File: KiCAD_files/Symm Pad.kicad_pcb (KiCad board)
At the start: 2 copper layers, 21 parts, among them J1 0.91"_OLED_Display, SW1 SW_Push, SW2 SW_Push, SW3 SW_Push, SW4 SW_Push, SW5 SW_Push, SW6 SW_Push, SW7 RotaryEncoder_Switch, U1 XIAO-RP2040-DIP

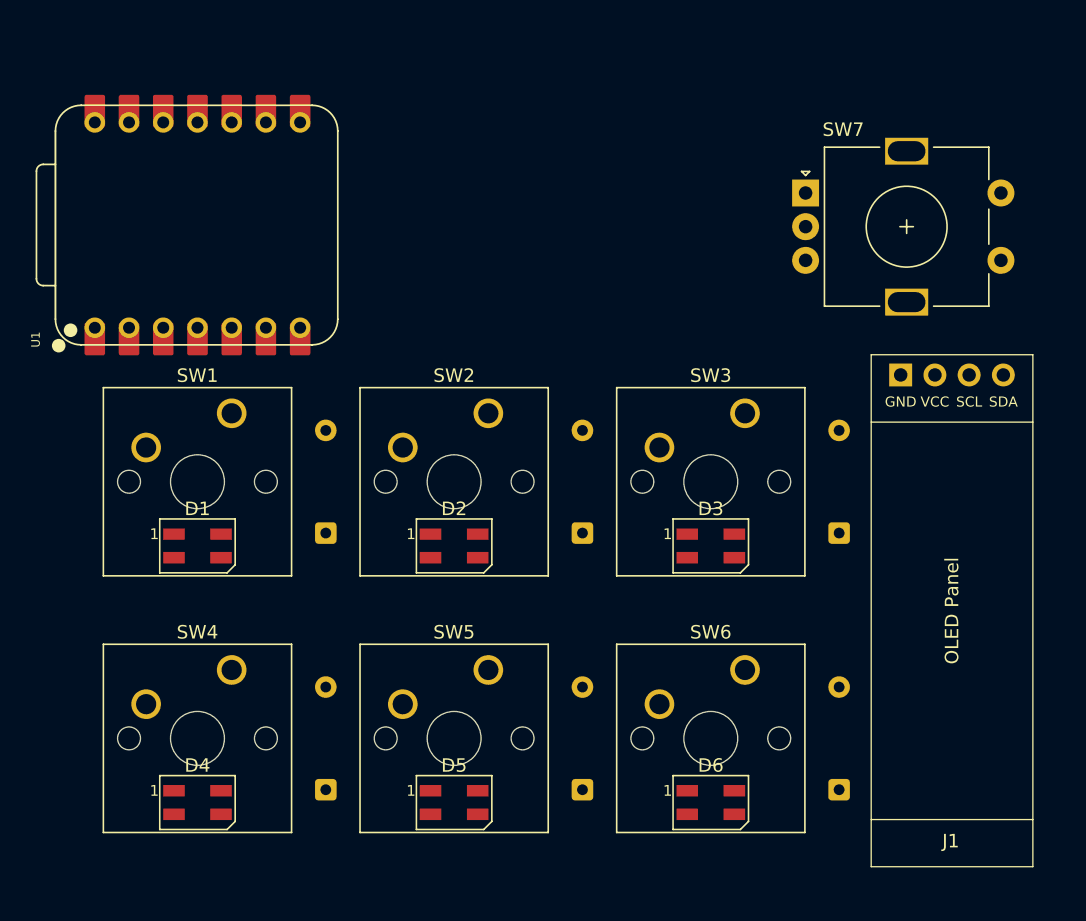
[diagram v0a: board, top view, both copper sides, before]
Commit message: Completed the PCB
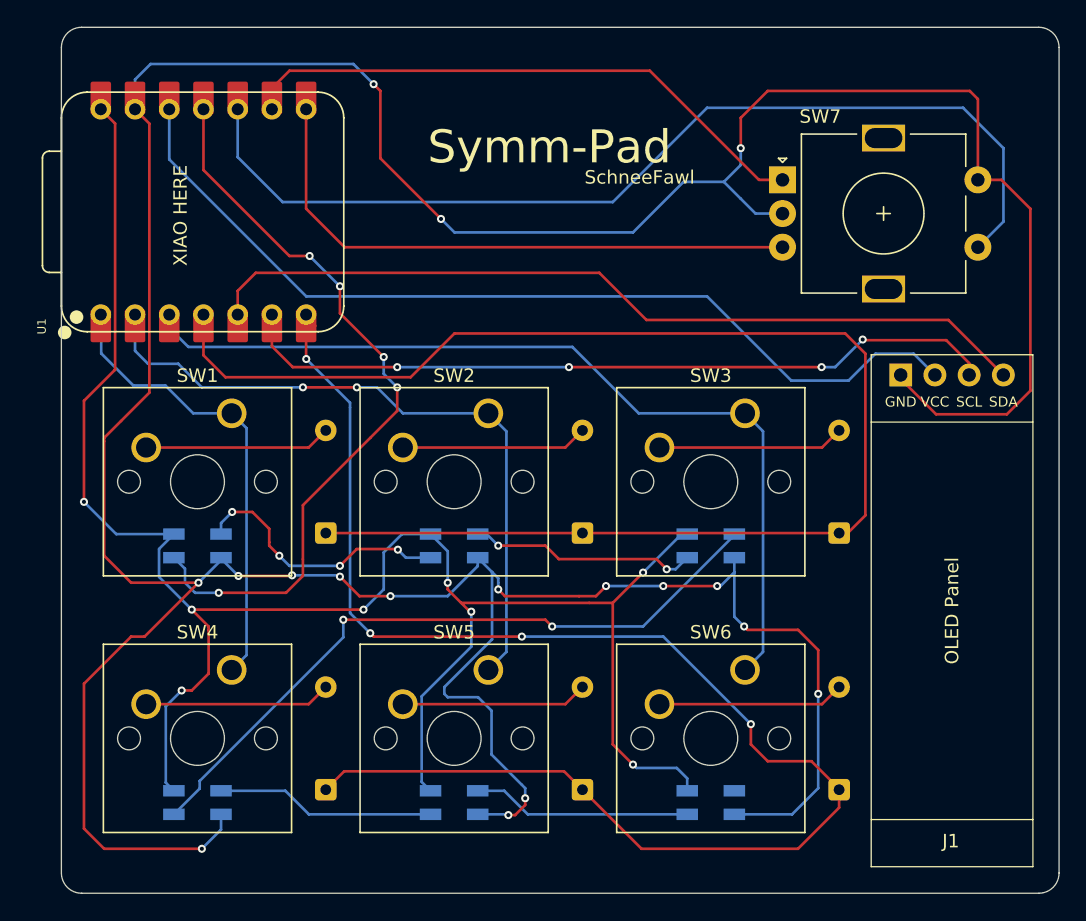
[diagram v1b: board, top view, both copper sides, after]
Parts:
- D1, D2, D3, D4, D5, D6: moved to B.Cu
- moved SW7 1.97 mm to (110.1, 27.6)
- moved U1 1.07 mm to (67.1, 30.0)
- turned D1 to 180 degrees
- turned D2 to 180 degrees
- turned D3 to 180 degrees
- turned D4 to 180 degrees
- turned D5 to 180 degrees
- turned D6 to 180 degrees
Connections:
- D10 pad 1: Row  1 -> Row 1
- D11 pad 1: Row  1 -> Row 1
- D12 pad 1: Row  1 -> Row 1
- D7 pad 1: Row  0 -> Row 0
- D8 pad 1: Row  0 -> Row 0
- D9 pad 1: Row  0 -> Row 0
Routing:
- net GND: track 0.00 -> 300.2 mm, vias 0 -> 17
- net +5V: track 0.00 -> 141.9 mm, vias 0 -> 8
- net Row 1: track 0.00 -> 110.5 mm, vias 0 -> 4
- net Row 0: track 0.00 -> 106.6 mm
- net Net-(U1-GPIO4/MISO): track 0.00 -> 74.1 mm
- net +3V3: track 0.00 -> 68.8 mm
- net Col 2: track 0.00 -> 66.5 mm
- net Net-(J1-Pin_4): track 0.00 -> 62.3 mm
- net Net-(J1-Pin_3): track 0.00 -> 56.4 mm, vias 0 -> 4
- net Net-(D1-DIN): track 0.00 -> 56.2 mm, vias 0 -> 5
- net Net-(D3-DOUT): track 0.00 -> 51.8 mm, vias 0 -> 2
- net Col 1: track 0.00 -> 51.0 mm, vias 0 -> 2
- net Net-(U1-GPIO1/RX): track 0.00 -> 43.9 mm
- net Net-(U1-GPIO2/SCK): track 0.00 -> 43.4 mm
- net Col 0: track 0.00 -> 33.9 mm
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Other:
- board outline added: 74 x 64.3 mm
- board text added: "SchneeFawl"
- board text added: "Symm-Pad"
- board text added: "XIAO HERE"
